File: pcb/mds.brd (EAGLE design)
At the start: 47.6 x 40.6 mm, 50 parts, among them IC1 MAX1555, M1 ELECTRET_MICROPHON-F6035AP, Q1 CSTCR6M00G53Z, U2 ISD1900ISD1932, U5 ATMEGA328

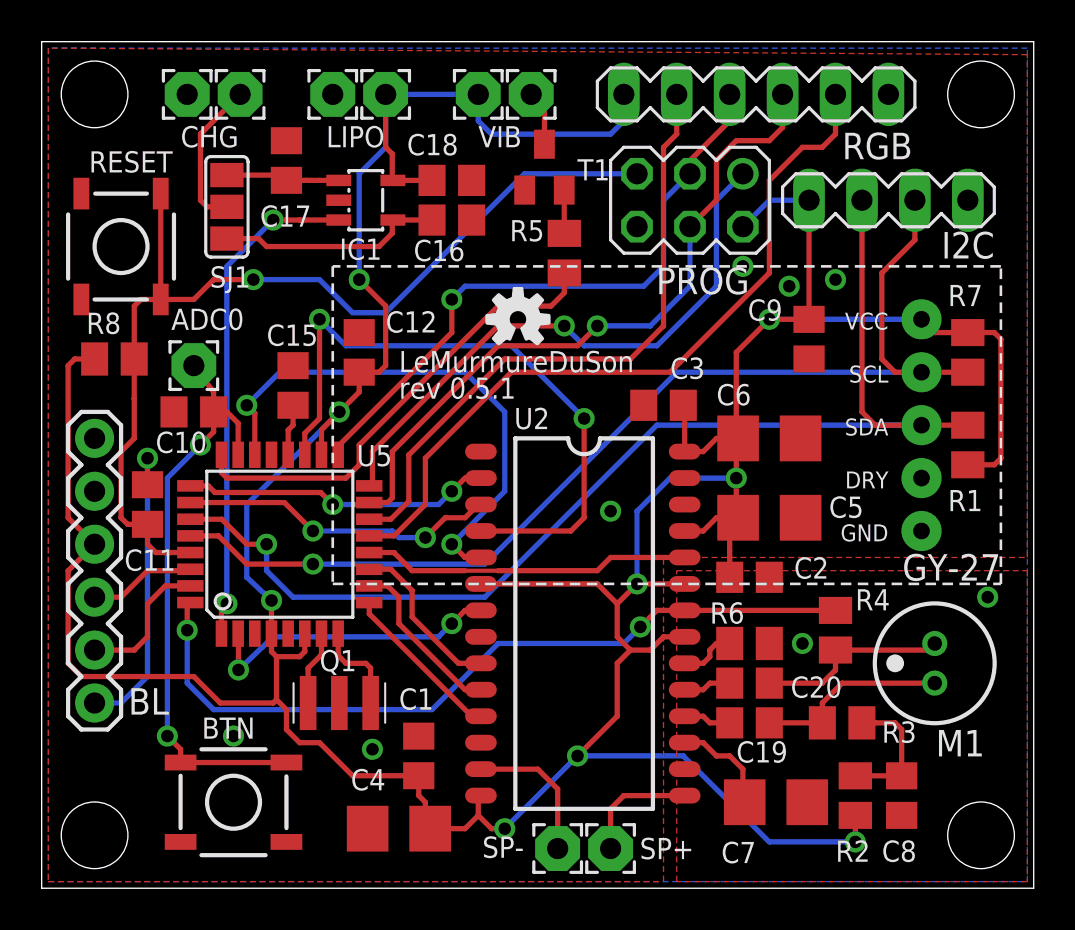
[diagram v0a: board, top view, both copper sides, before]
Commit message: PCB Version 0.6.2
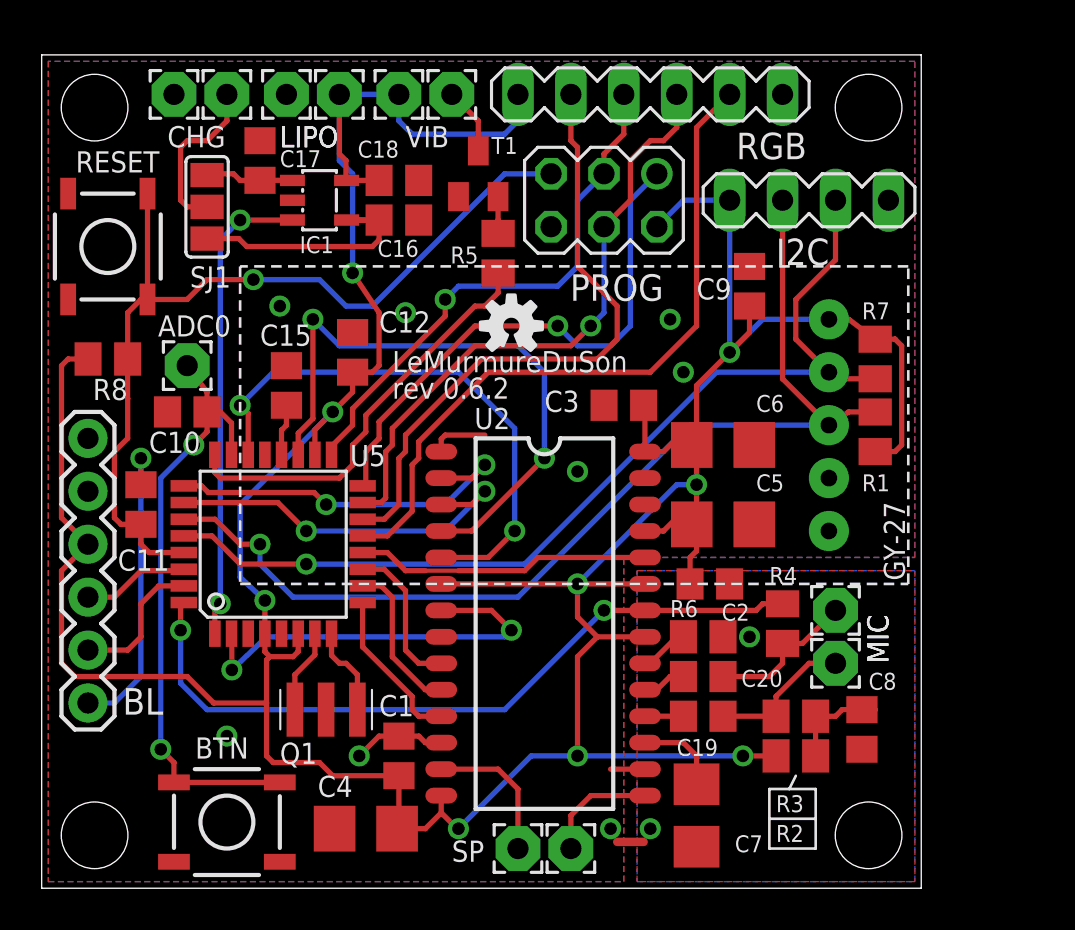
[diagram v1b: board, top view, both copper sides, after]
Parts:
- removed M1: ELECTRET_MICROPHON-F6035AP, microphon:F6035AP
- added MIC+, MIC-: (no value), wirepad:2,15/1,0
- moved RGB 5.08 mm to (29.2, 38.1)
- moved R1 4.49 mm to (40.0, 21.9)
- moved R7 4.46 mm to (40.0, 25.4)
- moved U$13 4.45 mm to (41.6, 29.8)
- moved PROG 4.13 mm to (27.0, 33.0)
- moved C7 3.86 mm to (31.4, 3.49), turned to 270 degrees
- moved C9 3.82 mm to (34.0, 28.9), turned to 270 degrees
- moved I2C 3.81 mm to (36.8, 33.0)
- moved MOT- 3.81 mm to (19.7, 38.1)
- moved MOT+ 3.81 mm to (17.1, 38.1)
- moved C8 3.70 mm to (39.4, 7.62)
- moved R2 3.43 mm to (36.2, 6.35), turned to 180 degrees
- moved T1 3.19 mm to (21.0, 34.3)
- moved R5 3.18 mm to (21.9, 30.5)
- moved R4 2.56 mm to (35.6, 12.7)
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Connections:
- net N$2: now also MIC+.1; no longer M1.1
- net N$3: now also MIC-.1; no longer M1.2
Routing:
- net VCC: track 208.3 -> 195.5 mm
- net GND: track 0.00 -> 10.2 mm, vias 8 -> 10
- net SDA: track 56.3 -> 50.6 mm
- net M5: track 14.5 -> 19.7 mm
- net SCL: track 52.1 -> 47.4 mm
- net RST: track 48.2 -> 43.9 mm
- net SCK: track 30.1 -> 25.9 mm
- net MOSI: track 33.0 -> 29.4 mm
- net M1: track 14.8 -> 18.0 mm
- net M2: track 15.3 -> 18.2 mm
- net VIBRATOR: track 23.3 -> 20.5 mm
- net SI: track 36.2 -> 33.7 mm
- net N$2: track 9.29 -> 7.01 mm
- net MISO: track 28.3 -> 26.1 mm
- net N$3: track 9.29 -> 7.28 mm
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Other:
- board size 47.6 x 40.6 mm -> 42.2 x 40 mm
- board text added: "DRY"
- board text added: "DTR"
- board text added: "GND"
- board text added: "I2C"
- board text added: "MIC"
- board text added: "Max 5V"
- board text added: "PROG"
- board text added: "RGB"
- board text added: "RXI"
- board text added: "SCL"
- board text added: "SDA"
- board text added: "SP"
- board text added: "SPEAKER"
- board text added: "TXO"
- board text added: "VCC"
- board text added: "VIBRATOR"
- board text added: "rev 0.6.2"
- board text removed: "rev 0.5.1"
